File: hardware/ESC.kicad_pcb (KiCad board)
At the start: 4 copper layers, 60 x 25 mm, 83 parts, among them J1 +, J2 -, J3 Conn_01x03, J4 +, J5 +, J6 +, J7 Conn_01x03, Q1 AGM60P30AP, Q2 AGM60P30AP, Q3 AGM60P30AP, Q4 AGM60P30AP, Q5 AGM60P30AP, Q6 AGM60P30AP, Q7 AGM60P30A, U1 DRV8323RSRGZR, U2 STM32G431CBTx, Y1 X322516MLB4SI

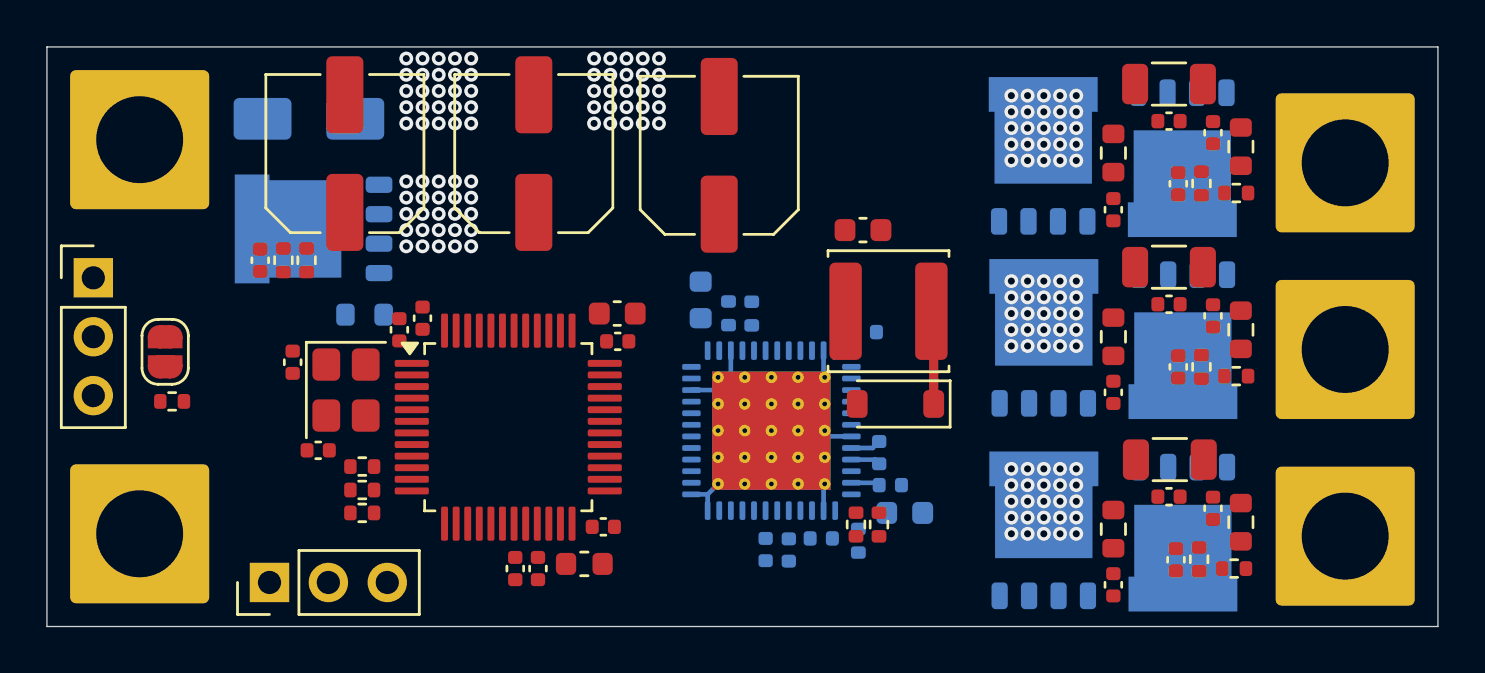
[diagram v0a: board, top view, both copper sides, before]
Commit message: started routing schematic
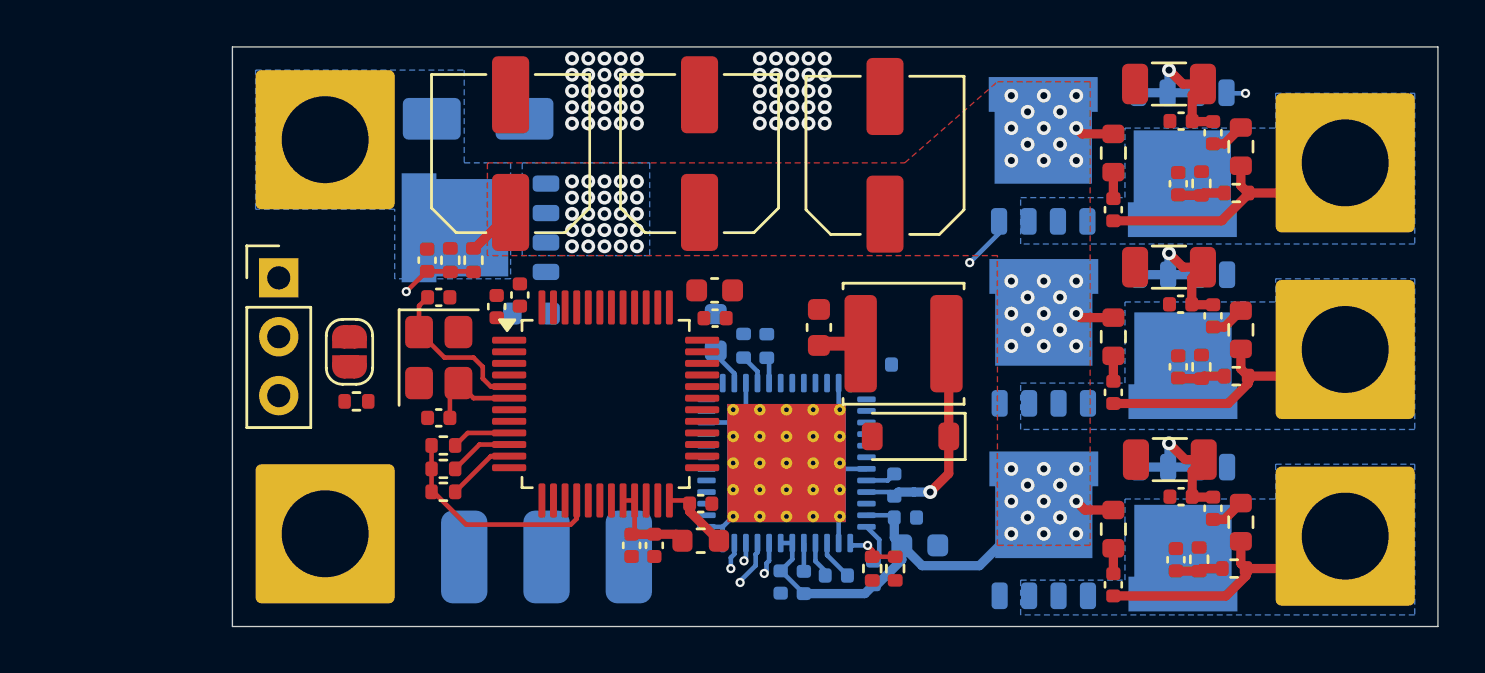
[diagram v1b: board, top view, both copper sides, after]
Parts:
- added J8: +, Connector_Wire:SolderWirePad_1x01_SMD_2x4mm, B.Cu at (151.6, 107.0)
- added J9: +, Connector_Wire:SolderWirePad_1x01_SMD_2x4mm, B.Cu at (155.1, 107.0)
- J3: value Conn_01x03 -> +; footprint Connector_PinHeader_2.54mm:PinHeader_1x03_P2.54mm_Vertical -> Connector_Wire:SolderWirePad_1x01_SMD_2x4mm; moved to B.Cu
- moved J3 8.47 mm to (148.0, 107.0), turned to 0 degrees
- moved J1 8.00 mm to (142.0, 89.0)
- moved J2 8.00 mm to (142.0, 106.0)
- moved J7 8.00 mm to (140.0, 95.0)
- moved JP1 7.95 mm to (143.1, 98.2)
- moved R20 7.95 mm to (143.3, 100.3)
- moved D2 7.30 mm to (148.6, 88.1)
- moved Q7 7.20 mm to (148.8, 92.8)
- moved R13 7.20 mm to (150.9, 96.5)
- moved C32 7.20 mm to (146.4, 94.2)
- moved R24 7.20 mm to (148.4, 94.2)
- moved R25 7.20 mm to (147.4, 94.2)
- moved C18 7.15 mm to (166.2, 89.7)
- moved C19 7.15 mm to (158.2, 89.6)
- moved C20 7.15 mm to (150.0, 89.6)
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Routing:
- net /MOTOR_A: track 0.00 -> 55.4 mm, vias 0 -> 1
- net /SPA: track 0.00 -> 42.3 mm, vias 0 -> 2
- net /GLA: track 0.00 -> 38.2 mm, vias 0 -> 2
- net VBUS: track 1.24 -> 26.4 mm, vias 100 -> 64
- net /GHA: track 0.00 -> 22.3 mm, vias 0 -> 2
- net /MOTOR_C: track 0.00 -> 12.5 mm
- net /MOTOR_B: track 0.00 -> 12.5 mm
- net /VIRTUAL_N: track 0.00 -> 9.69 mm
- net /SPC: track 0.00 -> 8.08 mm, vias 0 -> 1
- net /SPB: track 0.00 -> 7.92 mm, vias 0 -> 1
- net /HSE_IN: track 0.00 -> 6.72 mm
- net /BEMF_C: track 0.00 -> 5.02 mm
- net +3.3V: track 0.00 -> 4.88 mm
- net /BEMF_B: track 0.00 -> 4.81 mm
- net /BEMF_A: track 0.00 -> 4.59 mm
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- added copper zone on B.Cu, net /MOTOR_A
- added copper zone on B.Cu, net /MOTOR_B
- added copper zone on B.Cu, net /MOTOR_C
- added copper zone on B.Cu, net Net-(D2-A2)
- added copper zone on B.Cu, net VBUS
- added copper zone on F.Cu, net VBUS
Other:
- board size 60 x 25 mm -> 52 x 25 mm
